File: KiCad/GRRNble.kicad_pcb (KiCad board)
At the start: 2 copper layers, 28 x 36 mm, 29 parts, among them J1 JST_SH_06, J2 JST_SH_04, SW1 SW_Push, SW2 SW_Push, SW3 SW_Push, U1 R5F100LJAFB, U2 BUZZER, U3 SSD1306, Y1 32.768k

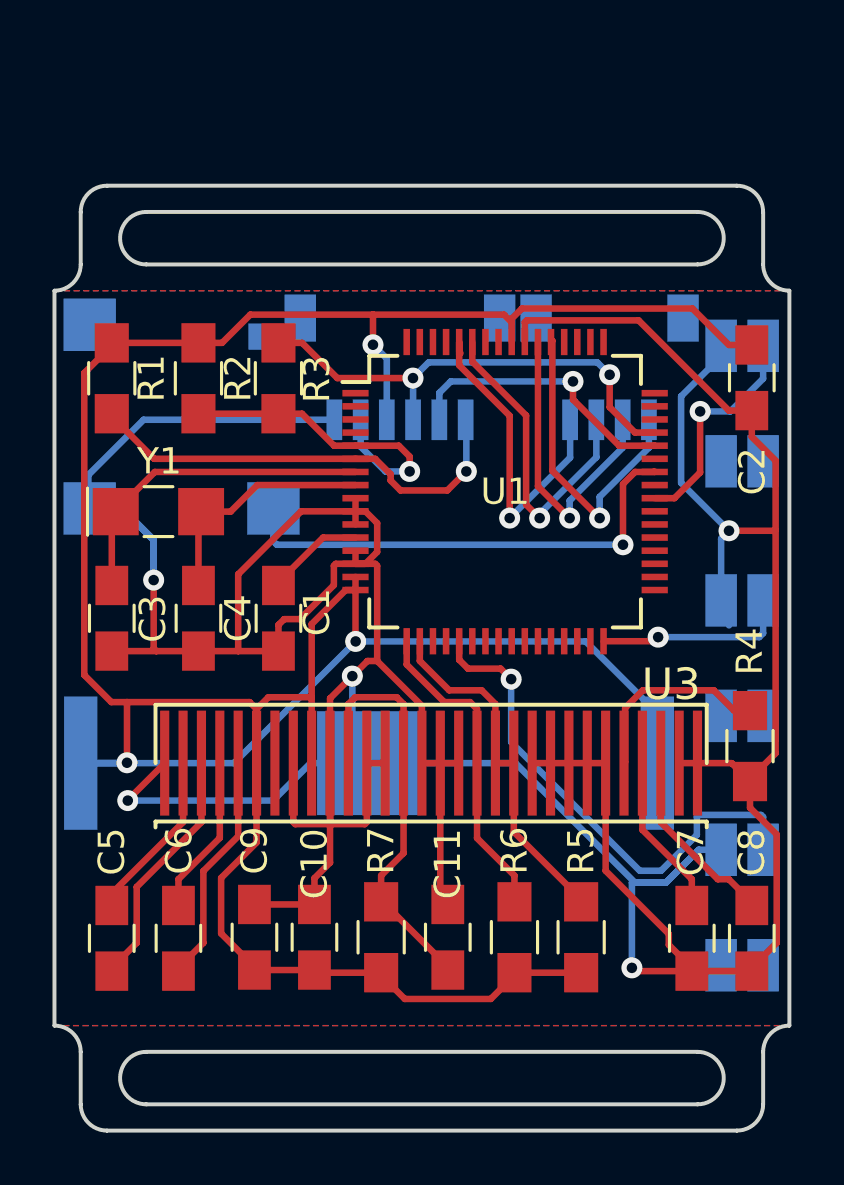
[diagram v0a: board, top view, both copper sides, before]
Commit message: WIP (PCB)
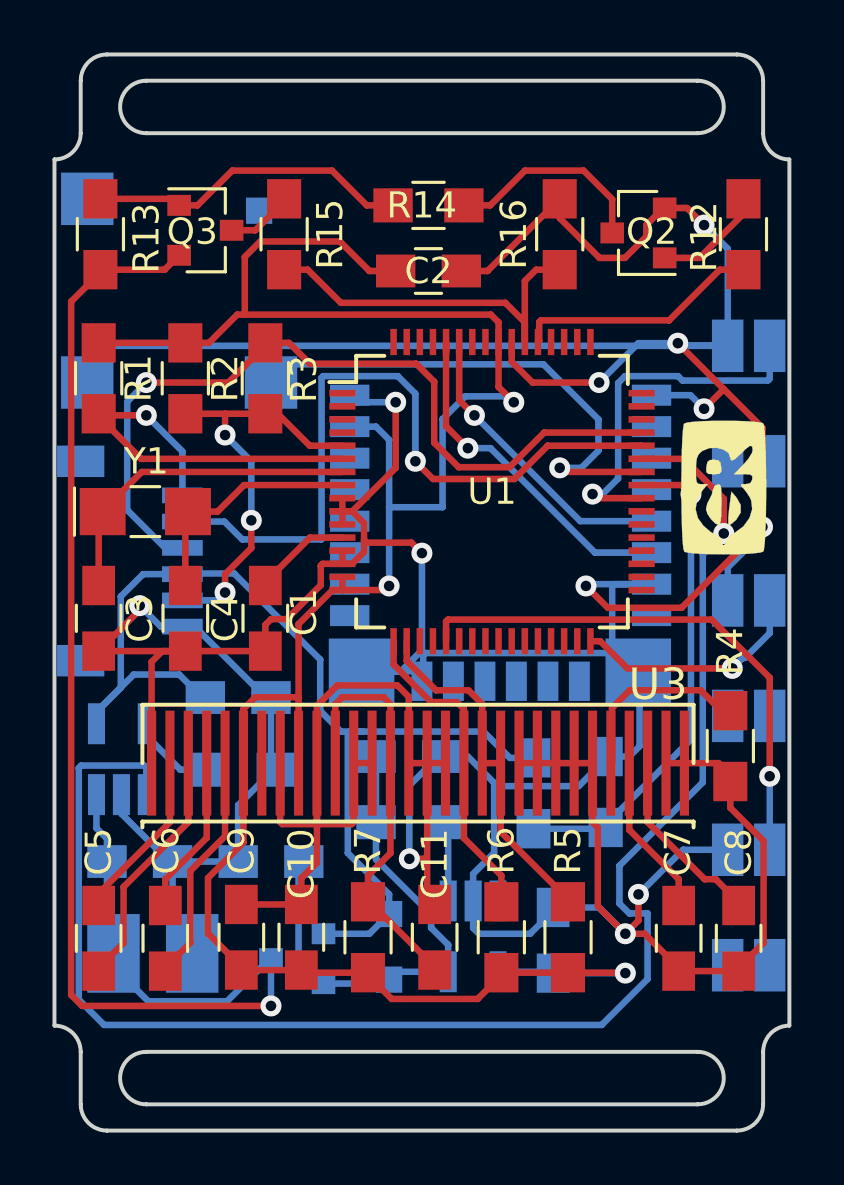
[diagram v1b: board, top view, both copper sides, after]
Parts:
- removed J2: JST_SH_04, JST-SH:JST-SM-04B-SRSS-TB
- added C12: 4.7uF, Capacitors_SMD:C_0805_HandSoldering, B.Cu at (102.2, 104.2)
- added C13: 4.7uF, Capacitors_SMD:C_0805_HandSoldering, B.Cu at (98.5, 110.4)
- added C14: 1.0uF, Capacitors_SMD:C_0805_HandSoldering, B.Cu at (103.5, 110.4)
- added C15: 0.1uF, Capacitors_SMD:C_0805_HandSoldering, B.Cu at (108.8, 106.4)
- added C16: 1.0uF, Capacitors_SMD:C_0805_HandSoldering, B.Cu at (114.2, 113.4)
- added D1: CUS10F30, Diodes_SMD:D_SOD-323_HandSoldering, B.Cu at (108.0, 113.7)
- added Q1: DMG3415U, TO_SOT_Packages_SMD:SOT-23, B.Cu at (104.5, 114.1)
- added Q2: BSS138, TO_SOT_Packages_SMD:SOT-23, F.Cu at (117.5, 86.5)
- added Q3: DMG3415U, TO_SOT_Packages_SMD:SOT-23, F.Cu at (101.0, 86.3)
- added R10: 47k, Resistors_SMD:R_0805_HandSoldering, B.Cu at (116.2, 107.8)
- added R11: 100k, Resistors_SMD:R_0805_HandSoldering, B.Cu at (108.8, 108.9)
- added R12: 100R, Resistors_SMD:R_0805_HandSoldering, F.Cu at (121.5, 86.5)
- added R13: 10k, Resistors_SMD:R_0805_HandSoldering, F.Cu at (97.0, 86.5)
- added R14: 100R, Resistors_SMD:R_0805_HandSoldering, F.Cu at (109.5, 85.4)
- added R15: 7K5, Resistors_SMD:R_0805_HandSoldering, F.Cu at (104.0, 86.5)
- added R16: 2K7, Resistors_SMD:R_0805_HandSoldering, F.Cu at (114.5, 86.5)
- added R8: 22k, Resistors_SMD:R_0805_HandSoldering, B.Cu at (102.3, 106.9)
- added R9: 47k, Resistors_SMD:R_0805_HandSoldering, B.Cu at (113.5, 107.8)
- added U4: MCP73831, TO_SOT_Packages_SMD:SOT-23-5_HandSoldering, B.Cu at (97.8, 106.5)
- added U5: RN4020, library:RN4020, B.Cu at (118.0, 103.5)
- added U6: NJM2865F33, TO_SOT_Packages_SMD:SOT-23-5_HandSoldering, B.Cu at (111.2, 113.2)
- BT1: footprint Battery_Holders:Keystone_3034_1x20mm-CoinCell -> misc:BatteryPad
- G***: moved to F.Cu
- moved G*** 17.6 mm to (120.8, 96.2), turned to 90 degrees
- moved C2 13.0 mm to (109.5, 87.9), turned to 0 degrees
- moved J1 12.5 mm to (98.2, 98.9), turned to 270 degrees
- moved BT1 10.0 mm to (99.0, 112.4)
- moved U2 4.80 mm to (100.0, 88.7)
- moved R4 0.75 mm to (121.0, 106.0)
- moved C1 0.50 mm to (103.3, 101.1)
- moved C10 0.50 mm to (104.7, 113.3)
- moved C11 0.50 mm to (109.7, 113.3)
- moved C3 0.50 mm to (96.9, 101.1)
- moved C4 0.50 mm to (100.2, 101.1)
- moved C5 0.50 mm to (96.9, 113.3)
- moved C6 0.50 mm to (99.5, 113.3)
- moved C7 0.50 mm to (119.0, 113.3)
- moved C8 0.50 mm to (121.3, 113.3)
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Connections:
- BT1 pad 1: +3V3 -> +BATT
- J1 pad 4: +3V3 -> Net-(C12-Pad1)
- J1 pad M1: Net-(J1-PadM1) -> (no net)
- J1 pad M2: Net-(J1-PadM2) -> (no net)
- U1 pad 1: Net-(U1-Pad1) -> (no net)
- U1 pad 19: Net-(U1-Pad19) -> (no net)
- U1 pad 2: Net-(U1-Pad2) -> (no net)
- U1 pad 20: Net-(U1-Pad20) -> (no net)
- U1 pad 22: Net-(U1-Pad22) -> (no net)
- U1 pad 23: Net-(U1-Pad23) -> (no net)
- U1 pad 24: Net-(U1-Pad24) -> (no net)
- U1 pad 25: Net-(U1-Pad25) -> (no net)
- U1 pad 26: Net-(U1-Pad26) -> (no net)
- U1 pad 27: Net-(U1-Pad27) -> (no net)
- U1 pad 28: Net-(U1-Pad28) -> (no net)
- U1 pad 29: Net-(U1-Pad29) -> (no net)
- U1 pad 3: Net-(U1-Pad3) -> (no net)
- U1 pad 30: Net-(U1-Pad30) -> (no net)
- U1 pad 31: Net-(U1-Pad31) -> (no net)
- U1 pad 33: Net-(U1-Pad33) -> (no net)
- U1 pad 34: Net-(U1-Pad34) -> (no net)
- U1 pad 35: Net-(U1-Pad35) -> (no net)
- U1 pad 36: Net-(U1-Pad36) -> (no net)
- U1 pad 37: Net-(U1-Pad37) -> (no net)
- U1 pad 38: Net-(U1-Pad38) -> (no net)
- U1 pad 39: Net-(U1-Pad39) -> (no net)
- U1 pad 4: Net-(U1-Pad4) -> (no net)
- U1 pad 41: Net-(U1-Pad41) -> VDD
- U1 pad 43: Net-(U1-Pad43) -> STAT
- U1 pad 46: Net-(U1-Pad46) -> (no net)
- U1 pad 47: Net-(U1-Pad47) -> (no net)
- U1 pad 48: Net-(U1-Pad48) -> (no net)
- U1 pad 49: Net-(U1-Pad49) -> (no net)
- U1 pad 50: Net-(U1-Pad50) -> (no net)
- U1 pad 51: Net-(U1-Pad51) -> (no net)
- U1 pad 52: Net-(U1-Pad52) -> (no net)
- U1 pad 53: A1 -> BATT_ENABLE
- U1 pad 54: A0 -> BATT_LEVEL
- U1 pad 57: Net-(U1-Pad57) -> (no net)
- U1 pad 58: Net-(U1-Pad58) -> (no net)
- U1 pad 59: D8 -> D8/RXD
- U1 pad 60: D7 -> D7/TXD
- U1 pad 61: Net-(U1-Pad61) -> (no net)
- U1 pad 62: Net-(U1-Pad62) -> (no net)
- U1 pad 63: Net-(U1-Pad63) -> (no net)
- U1 pad 64: Net-(U1-Pad64) -> (no net)
- U2 pad 3: Net-(U2-Pad3) -> (no net)
- U2 pad 4: Net-(U2-Pad4) -> (no net)
- U3 pad 7: Net-(U3-Pad7) -> (no net)
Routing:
- net GND: track 196.8 -> 259.6 mm, vias 5 -> 12
- net STAT: track 0.00 -> 59.9 mm, vias 0 -> 1
- net +BATT: track 0.00 -> 55.0 mm, vias 0 -> 1
- net Net-(C12-Pad1): track 0.00 -> 41.4 mm
- net +3V3: track 120.8 -> 87.5 mm
- net +5V: track 0.00 -> 19.3 mm
- net VDD: track 0.00 -> 18.8 mm, vias 0 -> 1
- net RXD: track 10.8 -> 27.6 mm
- net BATT_LEVEL: track 0.00 -> 14.6 mm
- net D7/TXD: track 0.00 -> 13.4 mm, vias 0 -> 1
- net A1: track 12.7 -> 0.00 mm, vias 1 -> 0
- net TXD: track 18.6 -> 31.3 mm, vias 2 -> 1
- net D7: track 12.6 -> 0.00 mm, vias 1 -> 0
- net A0: track 12.4 -> 0.00 mm, vias 1 -> 0
- net D8: track 12.4 -> 0.00 mm, vias 1 -> 0
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- removed copper zone on B.Cu, net GND
- removed copper zone on F.Cu, net GND
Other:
- board size 28 x 36 mm -> 28 x 41 mm
